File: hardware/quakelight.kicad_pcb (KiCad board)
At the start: 4 copper layers, 40 x 60 mm, 64 parts, among them J1 USB_C_Receptacle_USB2.0, J10 Conn_01x02_MountingPin, J2 RJ45_Abracon_ARJP11A-MASA-B-A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, J3 EZmate-4, J4 Conn_01x03_MountingPin, J5 Conn_01x03_MountingPin, J6 Conn_01x03_MountingPin, J7 TC2030-IDC-NL, SW1 SW_Push, SW2 SW_Push, U1 TPS7A0333DBVR, U10 STM32H573RIVx, U3 KSZ8081RNA, U4 SN74LV1T125DBV, U5 SN74LV1T125DBV, U6 TPS2116DRL, U7 SN74LV1T125DBV, Y1 25MHz, Y2 32.768kHz

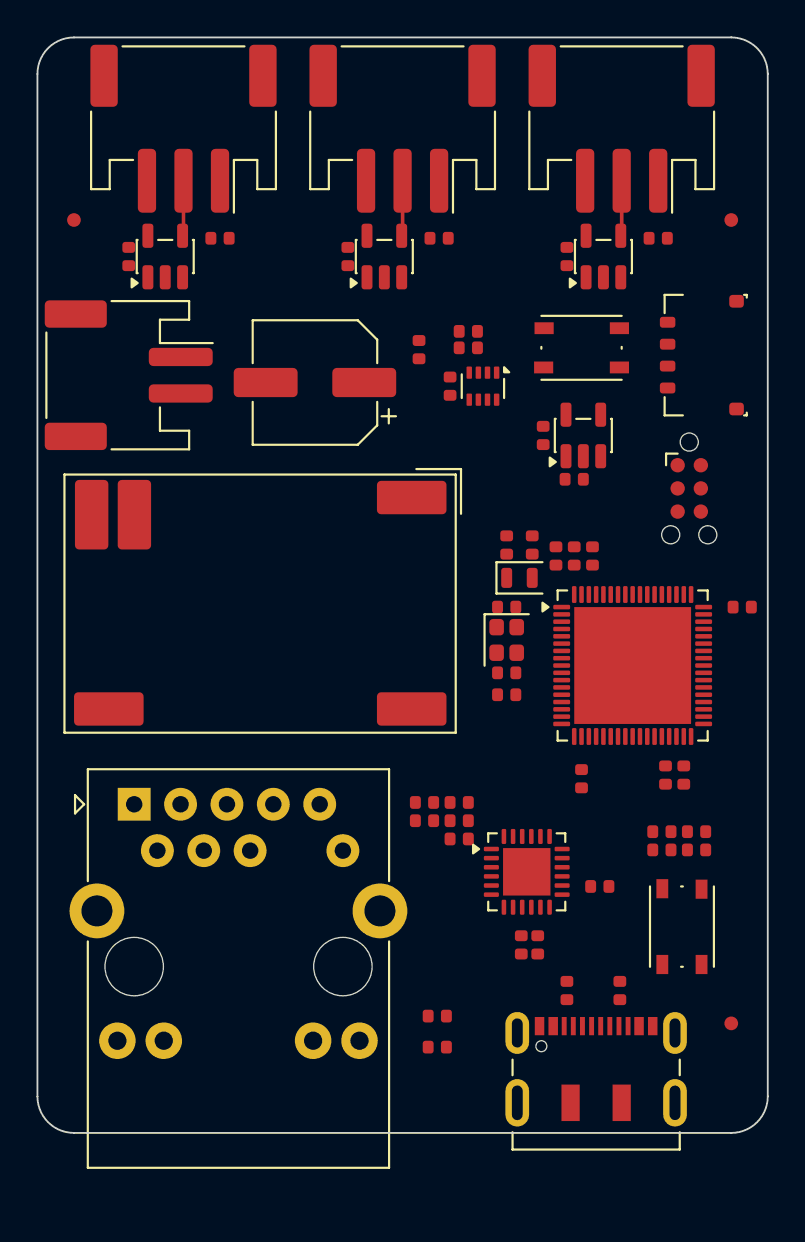
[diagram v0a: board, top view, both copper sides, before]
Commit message: wip
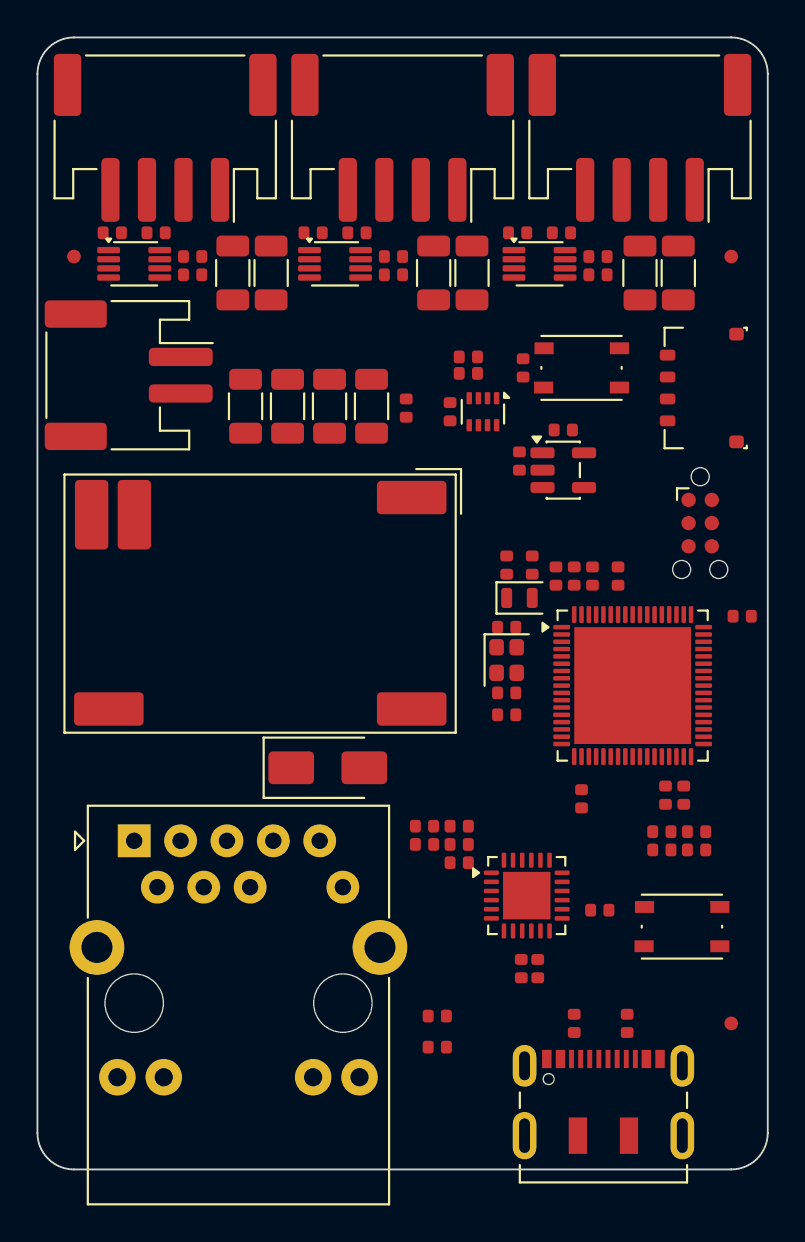
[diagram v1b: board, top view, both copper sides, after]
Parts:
- removed J6: Conn_01x03_MountingPin, Connector_JST:JST_PH_S3B-PH-SM4-TB_1x03-1MP_P2.00mm_Horizontal
- removed U7: SN74LV1T125DBV, Package_TO_SOT_SMD:SOT-23-5
- added C14: 100u, Capacitor_SMD:C_1206_3216Metric, F.Cu at (155.1, 92.9)
- added C15: 100u, Capacitor_SMD:C_1206_3216Metric, F.Cu at (143.8, 92.9)
- added C16: 100u, Capacitor_SMD:C_1206_3216Metric, F.Cu at (141.7, 92.9)
- added C20: 100n, balto:C_0402_Worthington, F.Cu at (124.1, 90.7)
- added C21: 100n, balto:C_0402_Worthington, F.Cu at (146.3, 90.7)
- added C22: 100n, balto:C_0402_Worthington, F.Cu at (135.1, 90.7)
- added C23: 100u, Capacitor_SMD:C_1206_3216Metric, F.Cu at (133.7, 100.2)
- added C24: 100u, Capacitor_SMD:C_1206_3216Metric, F.Cu at (136.0, 100.2)
- added C25: 100u, Capacitor_SMD:C_1206_3216Metric, F.Cu at (131.4, 100.2)
- added D3: SMAJ58A, Diode_SMD:D_SMA, F.Cu at (135.9, 120.0)
- added J9: PH, Connector_JST:JST_PH_S4B-PH-SM4-TB_1x04-1MP_P2.00mm_Horizontal, F.Cu at (127.0, 85.5)
- added R10: 100, balto:R_0402_Worthington, F.Cu at (128.5, 93.0)
- added R11: 100, balto:R_0402_Worthington, F.Cu at (139.5, 92.0)
- added R14: 100, balto:R_0402_Worthington, F.Cu at (139.5, 93.0)
- added R15: 100, balto:R_0402_Worthington, F.Cu at (150.7, 92.0)
- added R16: 100, balto:R_0402_Worthington, F.Cu at (150.7, 93.0)
- added R6: 0, balto:R_0402_Worthington, F.Cu at (151.8, 109.5)
- added R7: 1k, balto:R_0402_Worthington, F.Cu at (146.6, 98.1)
- added R8: 100, balto:R_0402_Worthington, F.Cu at (128.5, 92.0)
- added U8: SN74LVC2T45DCUR, Package_SO:VSSOP-8_2.3x2mm_P0.5mm, F.Cu at (125.3, 92.4)
- C13, C4, C8: value 10u -> 100u; footprint balto:C_0402_Worthington -> Capacitor_SMD:C_1206_3216Metric
- C19: footprint Capacitor_SMD:CP_Elec_6.3x7.7 -> Capacitor_SMD:C_1206_3216Metric
- J4, J5: value Conn_01x03_MountingPin -> PH; footprint Connector_JST:JST_PH_S3B-PH-SM4-TB_1x03-1MP_P2.00mm_Horizontal -> Connector_JST:JST_PH_S4B-PH-SM4-TB_1x04-1MP_P2.00mm_Horizontal
- U4, U5: value SN74LV1T125DBV -> SN74LVC2T45DCUR; footprint Package_TO_SOT_SMD:SOT-23-5 -> Package_SO:VSSOP-8_2.3x2mm_P0.5mm
- moved C8 23.4 mm to (130.7, 92.9), turned to -90 degrees
- moved J4 12.0 mm to (140.0, 85.5)
- moved C10 11.8 mm to (148.7, 90.7), turned to 180 degrees
- moved C6 11.6 mm to (137.5, 90.7), turned to 180 degrees
- moved C13 11.2 mm to (153.0, 92.9), turned to -90 degrees
- moved U4 9.31 mm to (136.3, 92.4), turned to 0 degrees
- moved U5 3.52 mm to (147.5, 92.4), turned to 0 degrees
- moved C4 3.38 mm to (132.8, 92.9), turned to -90 degrees
- moved C19 3.36 mm to (138.3, 100.2), turned to 90 degrees
- moved C3 3.28 mm to (140.2, 100.3)
- moved C1 3.16 mm to (146.4, 103.2), turned to -90 degrees
- moved U1 2.20 mm to (148.8, 103.7), turned to 0 degrees
- moved FID1 2.00 mm to (122.0, 92.0)
- moved FID3 2.00 mm to (158.0, 92.0)
- moved J2 2.00 mm to (125.3, 124.0)
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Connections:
- J4 pad 3: GND -> Net-(J4-Pin_3)
- J5 pad 3: GND -> Net-(J5-Pin_3)
- SW1 pad 1: /SW1 -> /BOOT0
- SW1 pad 2: GND -> +3V3
- U10 pad 45: unconnected-(U10-PA9-Pad45) -> /SPI2_SCK
- U10 pad 54: unconnected-(U10-PC10-Pad54) -> /SPI3_SCK
- U10 pad 57: unconnected-(U10-PB3(JTDO-Pad57) -> /SPI1_SCK
- U10 pad 62: GND -> /BOOT0
- U10 pad 63: unconnected-(U10-PB8-Pad63) -> /SW1
- U4 pad 1: GND -> +3V3
- U4 pad 2: /SPI1_MOSI -> /SPI2_SCK
- U4 pad 3: GND -> /SPI2_MOSI
- U4 pad 4: Net-(J4-Pin_2) -> GND
- U4 pad 5: +5V -> +3V3
- U5 pad 1: GND -> +3V3
- U5 pad 2: /SPI2_MOSI -> /SPI3_SCK
- U5 pad 3: GND -> /SPI3_MOSI
- U5 pad 4: Net-(J5-Pin_2) -> GND
- U5 pad 5: +5V -> +3V3
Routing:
- net Net-(J6-Pin_2): track 3.03 -> 0.00 mm
- net Net-(J5-Pin_2): track 3.03 -> 0.00 mm
- net Net-(J4-Pin_2): track 3.03 -> 0.00 mm
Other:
- board size 40 x 60 mm -> 40 x 62 mm
